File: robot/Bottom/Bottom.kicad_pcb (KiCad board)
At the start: 2 copper layers, 46 x 46 mm, 39 parts, among them M1 Stepper_Motor_bipolar, M2 Stepper_Motor_bipolar, U1 GP2S60, U2 GP2S60, U7 DRV8833PWP, U8 DRV8833PWP

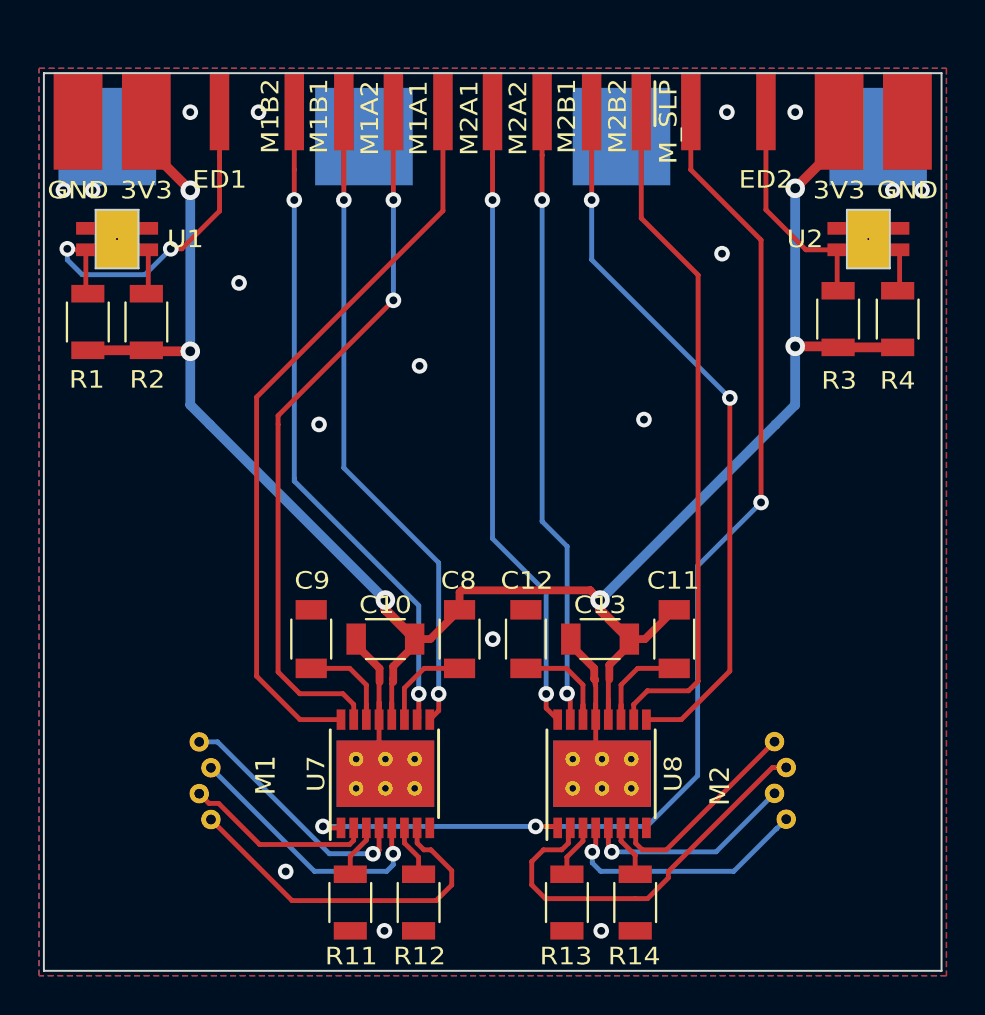
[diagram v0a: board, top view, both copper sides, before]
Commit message: Finisch bottom
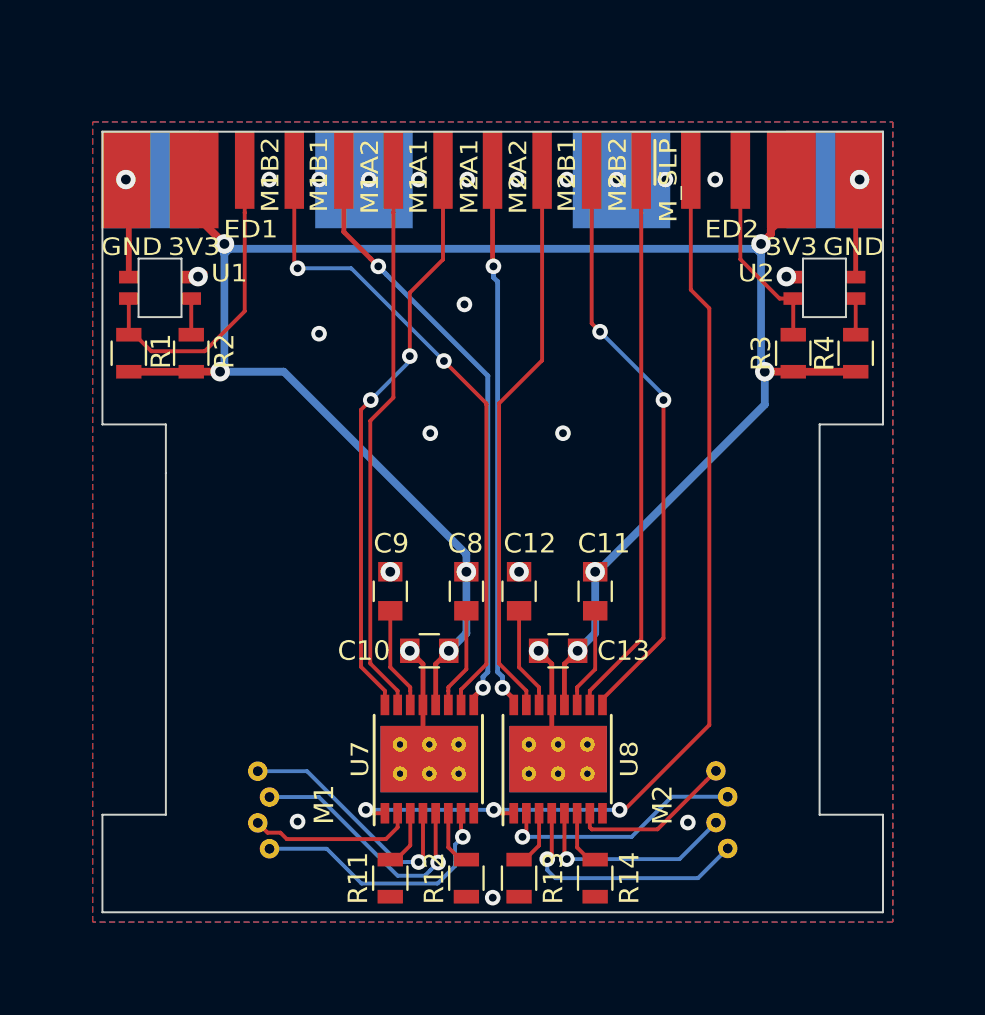
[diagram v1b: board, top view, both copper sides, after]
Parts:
- C10, C11, C12, C13, C8, C9: footprint Capacitors_SMD:C_1206 -> Capacitors_SMD:C_0805
- R1, R11, R12, R13, R14, R2, R3, R4: footprint Resistors_SMD:R_1206 -> Resistors_SMD:R_0805
- moved C11 4.73 mm to (178.2, 101.5)
- moved C9 4.73 mm to (167.8, 101.5)
- moved H12 3.87 mm to (188.3, 80.5)
- moved H13 3.87 mm to (154.2, 80.5)
- moved H14 3.87 mm to (191.8, 80.5)
- moved H15 3.87 mm to (157.7, 80.5)
- moved U2 3.36 mm to (189.8, 83.8)
- moved M1 3.35 mm to (161.2, 112.8)
- moved M2 3.35 mm to (184.8, 112.8)
- moved U1 3.33 mm to (155.8, 83.8)
- moved H6 3.27 mm to (185.7, 80.0)
- moved H5 3.27 mm to (160.3, 80.0)
- moved H18 3.11 mm to (155.4, 80.5)
- moved H19 3.11 mm to (190.6, 80.5)
- moved H1 3.00 mm to (170.4, 80.0)
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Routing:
- net /M1_~SLEEP: track 60.0 -> 50.4 mm
- net /M1_AIN1: track 38.2 -> 29.7 mm, vias 0 -> 2
- net /M1_AIN2: track 36.5 -> 28.5 mm, vias 2 -> 0
- net Net-(M2-Pad1): track 20.6 -> 12.7 mm, vias 0 -> 1
- net /M2_BIN2: track 35.0 -> 28.5 mm
- net /M2_BIN1: track 36.9 -> 30.5 mm
- net Net-(M1-Pad3): track 18.3 -> 13.5 mm, vias 0 -> 1
- net /M2_AIN1: track 32.6 -> 27.9 mm
- net +3V3: track 100.7 -> 104.7 mm, vias 6 -> 8
- net GND: track 22.4 -> 25.7 mm, vias 17 -> 25
- net /M2_AIN2: track 31.8 -> 28.9 mm, vias 2 -> 0
- net /M1_BIN1: track 33.4 -> 30.8 mm
- net Net-(H5-Pad1): track 18.4 -> 16.4 mm, vias 2 -> 0
- net Net-(M2-Pad3): track 10.4 -> 8.47 mm
- net Net-(H6-Pad1): track 11.7 -> 9.98 mm
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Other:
- board size 46 x 46 mm -> 40 x 40 mm
- net class Default: trace_width 0.25 -> 0.2
- net class Power: trace_width 0.5 -> 0.4
